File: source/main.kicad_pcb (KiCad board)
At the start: 2 copper layers, 85.6 x 54 mm, 62 parts, among them P1 USB_Type_C_Receptacle_16_pin

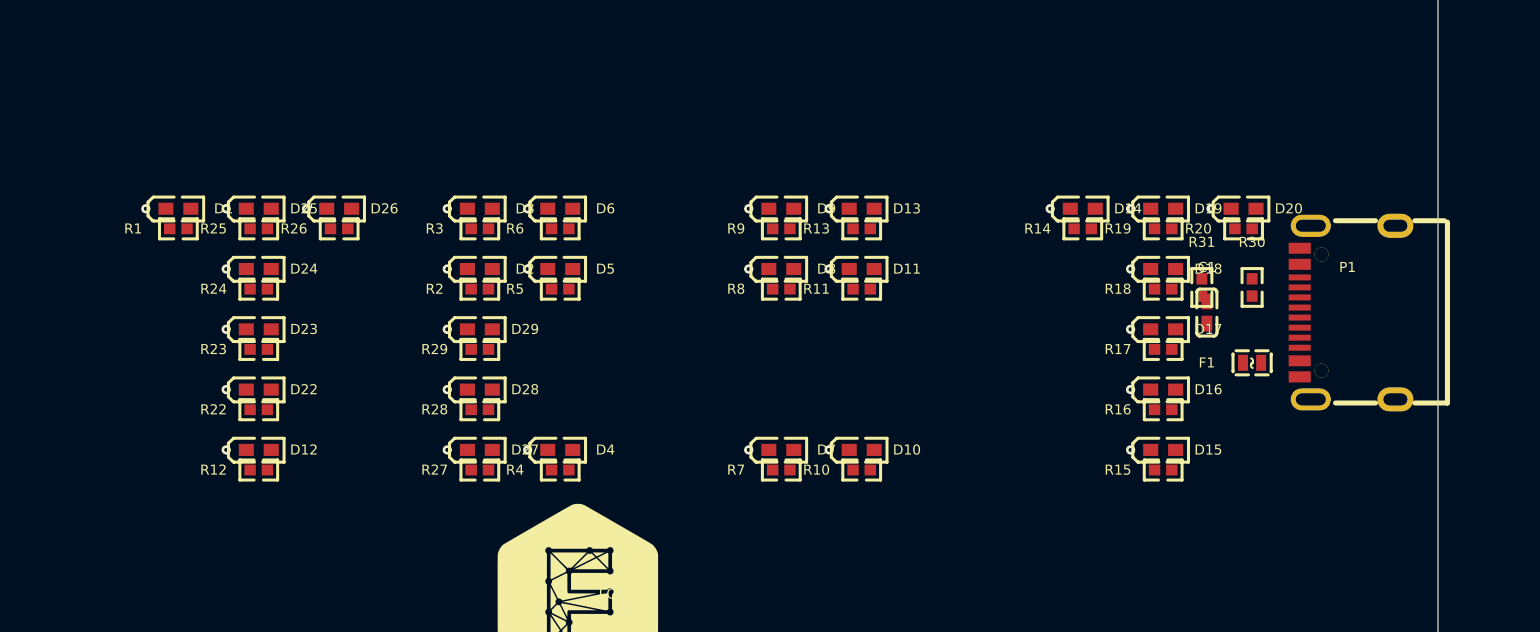
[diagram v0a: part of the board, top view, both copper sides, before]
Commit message: Rerun, only F, no connect
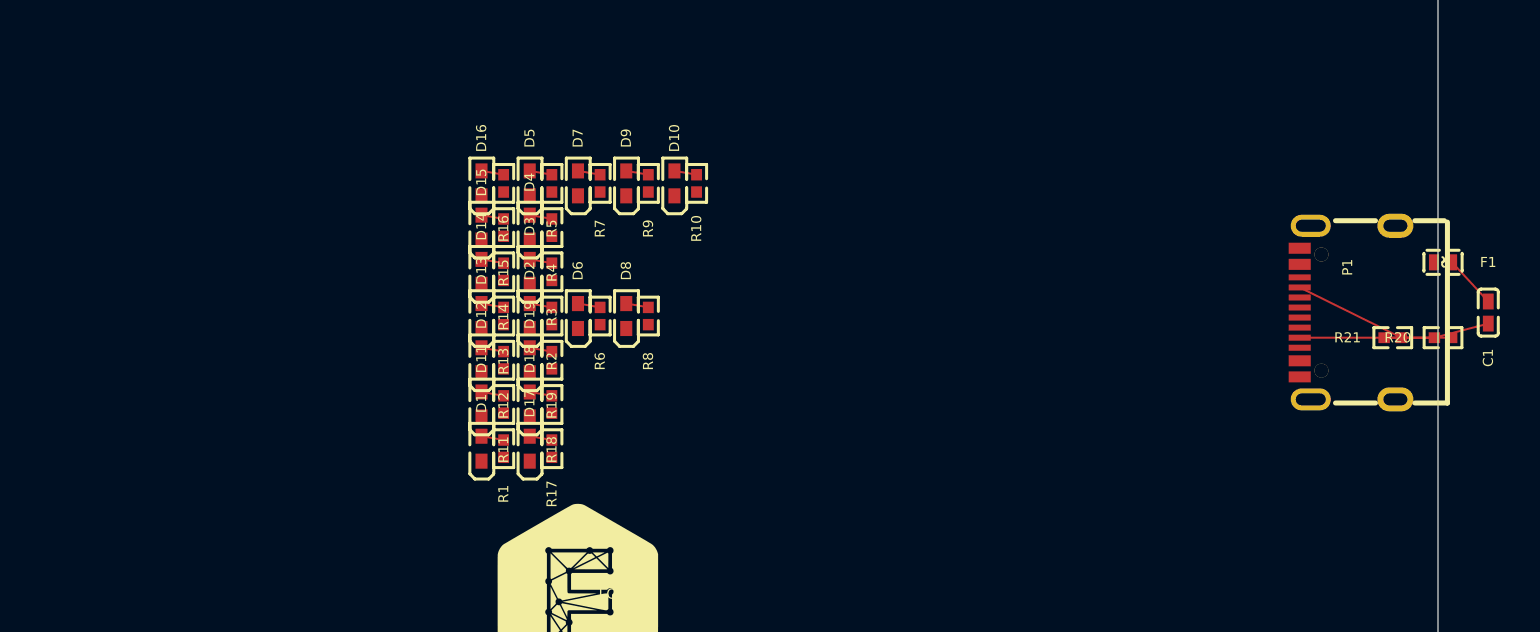
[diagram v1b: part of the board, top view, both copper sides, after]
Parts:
- removed D20, D22, D23, D24, D25, D26, D27, D28, D29: LED, lcsc:LED0402-R-RD_RED
- removed R22, R23, R24, R25, R26, R27, R28, R29: 100Ω, lcsc:R0402
- removed R30, R31: 5.1kΩ, lcsc:R0402
- added R21: 5.1kΩ, lcsc:R0402, F.Cu at (83.3, 28.2)
- R20: value 100Ω -> 5.1kΩ
- moved D15 35.7 mm to (38.0, 22.8), turned to 90 degrees
- moved D16 35.4 mm to (38.0, 20.6), turned to 90 degrees
- moved R15 35.0 mm to (39.1, 22.8), turned to -90 degrees
- moved R16 34.7 mm to (39.1, 20.6), turned to -90 degrees
- moved D19 32.4 mm to (40.4, 29.4), turned to 90 degrees
- moved D18 32.2 mm to (40.4, 31.6), turned to 90 degrees
- moved D17 32.1 mm to (40.4, 33.8), turned to 90 degrees
- moved R19 31.1 mm to (41.5, 29.4), turned to -90 degrees
- moved R18 31.0 mm to (41.5, 31.6), turned to -90 degrees
- moved R17 30.8 mm to (41.5, 33.8), turned to -90 degrees
- moved D14 30.1 mm to (38.0, 25.0), turned to 90 degrees
- moved R14 28.9 mm to (39.1, 25.0), turned to -90 degrees
- moved D11 20.1 mm to (38.0, 31.6), turned to 90 degrees
- moved D13 19.7 mm to (38.0, 27.2), turned to 90 degrees
- moved R1 19.5 mm to (39.1, 33.8), turned to -90 degrees
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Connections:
- P1 pad 4: P1-4-R30-1 -> P1-4-R20-1
- P1 pad 9: P1-9-R31-1 -> P1-9-R21-1
- R20 pad 1: D20-1-R20-1 -> P1-4-R20-1
- R20 pad 2: R20-2 -> gnd
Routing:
- net P1-4-R20-1: track 0.00 -> 7.56 mm
- net P1-9-R21-1: track 0.00 -> 5.64 mm
- net gnd: track 0.00 -> 5.27 mm
- net vbus: track 0.00 -> 2.65 mm
- net D8-1-R8-1: track 0.00 -> 1.12 mm
- net D3-1-R3-1: track 0.00 -> 1.12 mm
- net D2-1-R2-1: track 0.00 -> 1.12 mm
- net D19-1-R19-1: track 0.00 -> 1.12 mm
- net D14-1-R14-1: track 0.00 -> 1.12 mm
- net D13-1-R13-1: track 0.00 -> 1.12 mm
- net D12-1-R12-1: track 0.00 -> 1.12 mm
- net D9-1-R9-1: track 0.00 -> 1.12 mm
- net D5-1-R5-1: track 0.00 -> 1.12 mm
- net D4-1-R4-1: track 0.00 -> 1.12 mm
- net D18-1-R18-1: track 0.00 -> 1.12 mm
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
